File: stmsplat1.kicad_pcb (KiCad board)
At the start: 2 copper layers, 12 parts, among them CN1 C_Pack04, CN10 Conn_01x34_Male, CN7 Conn_01x20_Male, CN8 Conn_01x16_Male, CN9 Conn_01x30_Male, J1 Conn_Coaxial, J2 Conn_Coaxial, J3 Conn_Coaxial, U1 NUCLEO144-F746ZG, U2 SA630D

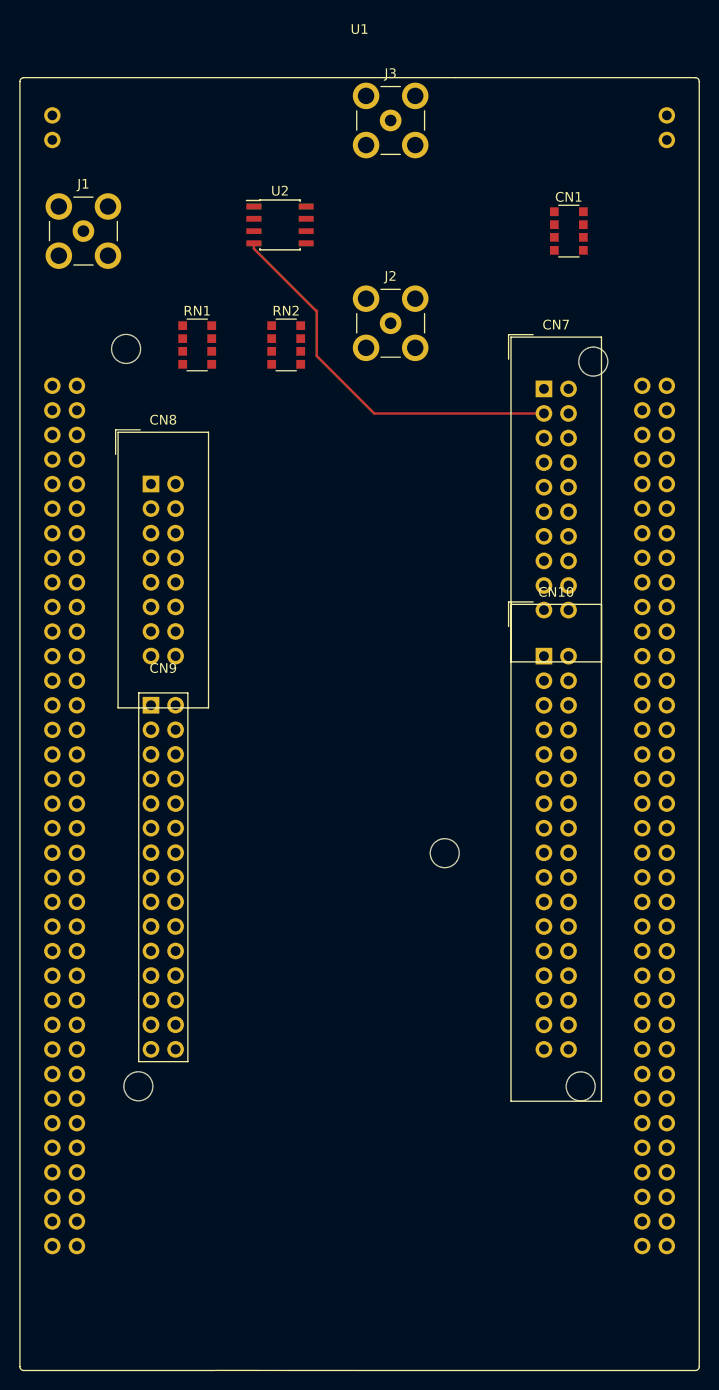
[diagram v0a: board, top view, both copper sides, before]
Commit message: Getting ready for proper start to project
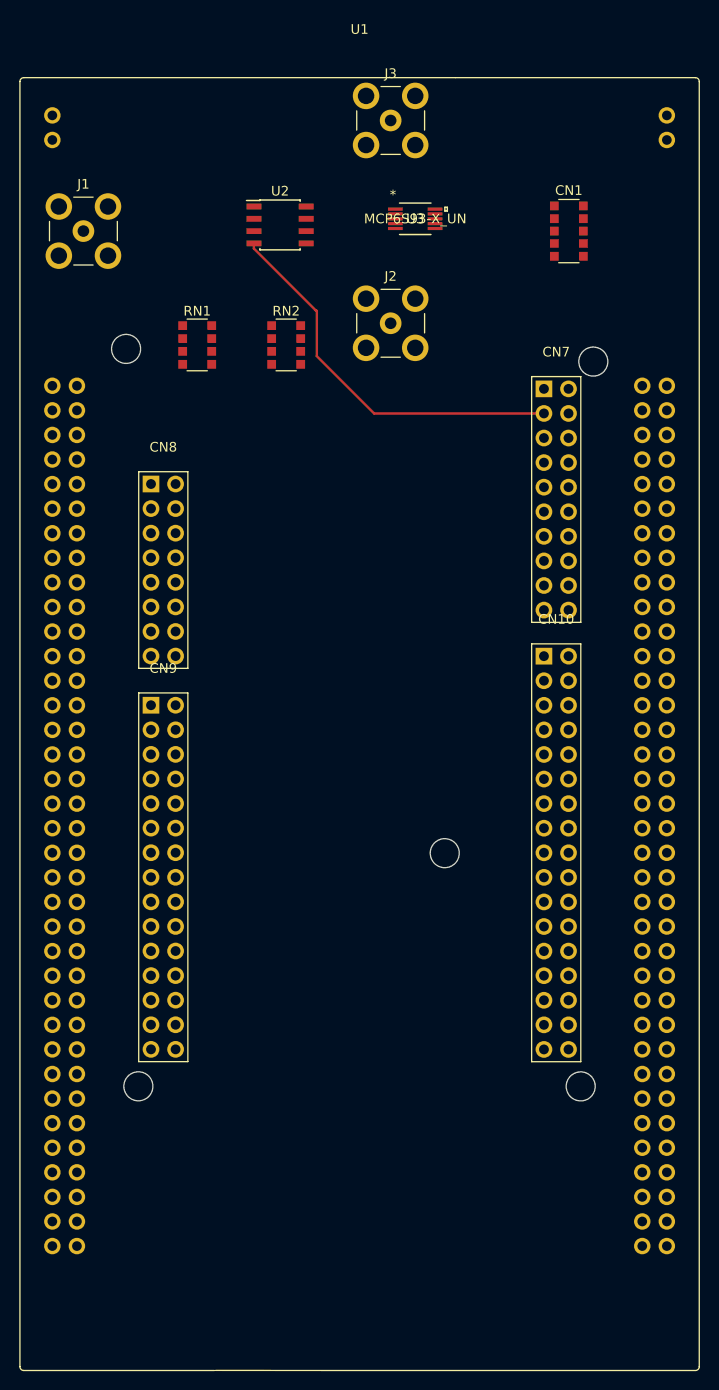
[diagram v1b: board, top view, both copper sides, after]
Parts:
- added U3: MCP6S93-X_UN, spatboard:MCP6S93-X&slash_UN, F.Cu at (95.9, 48.3)
- CN1: value C_Pack04 -> C_Pack04-c_pack04; footprint symbols:C_Array_Convex_4x1206 -> spatboard:C_Array_Convex_5x1206
- CN10: footprint Connector_IDC:IDC-Header_2x17_P2.54mm_Vertical -> spatboard:IDC-Pins_2x17_P2.54mm_Vertical
- CN7: footprint Connector_IDC:IDC-Header_2x10_P2.54mm_Vertical -> spatboard:IDC-Pins_2x10_P2.54mm_Vertical
- CN8: footprint Connector_IDC:IDC-Header_2x08_P2.54mm_Vertical -> spatboard:IDC-Pins_2x8_P2.54mm_Vertical
- U2: value SA630D -> SA630D-RF_Switch
